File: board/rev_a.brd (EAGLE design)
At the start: 56 x 25 mm, 19 parts, among them IC3 MCP2551, Q1 35A/25V/8.5mΩ

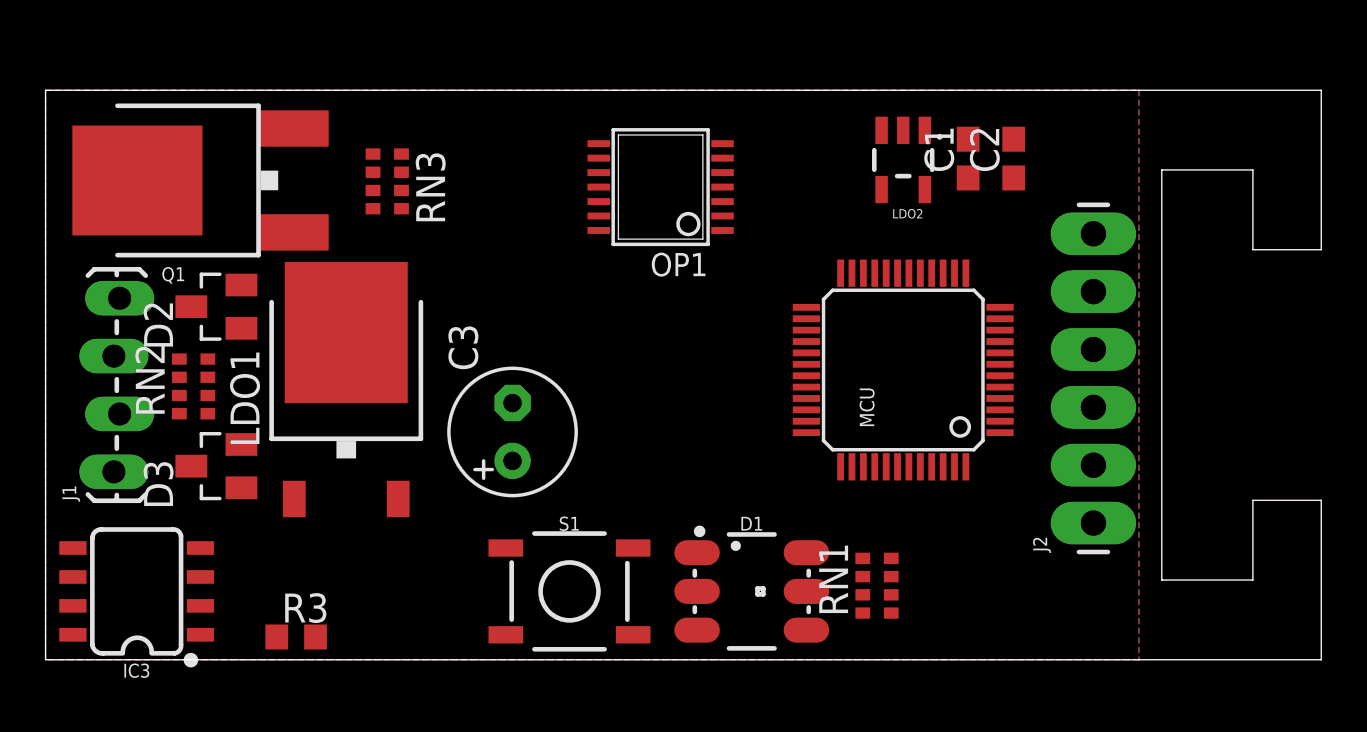
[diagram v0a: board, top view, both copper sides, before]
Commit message: [board] Testing a few configurations
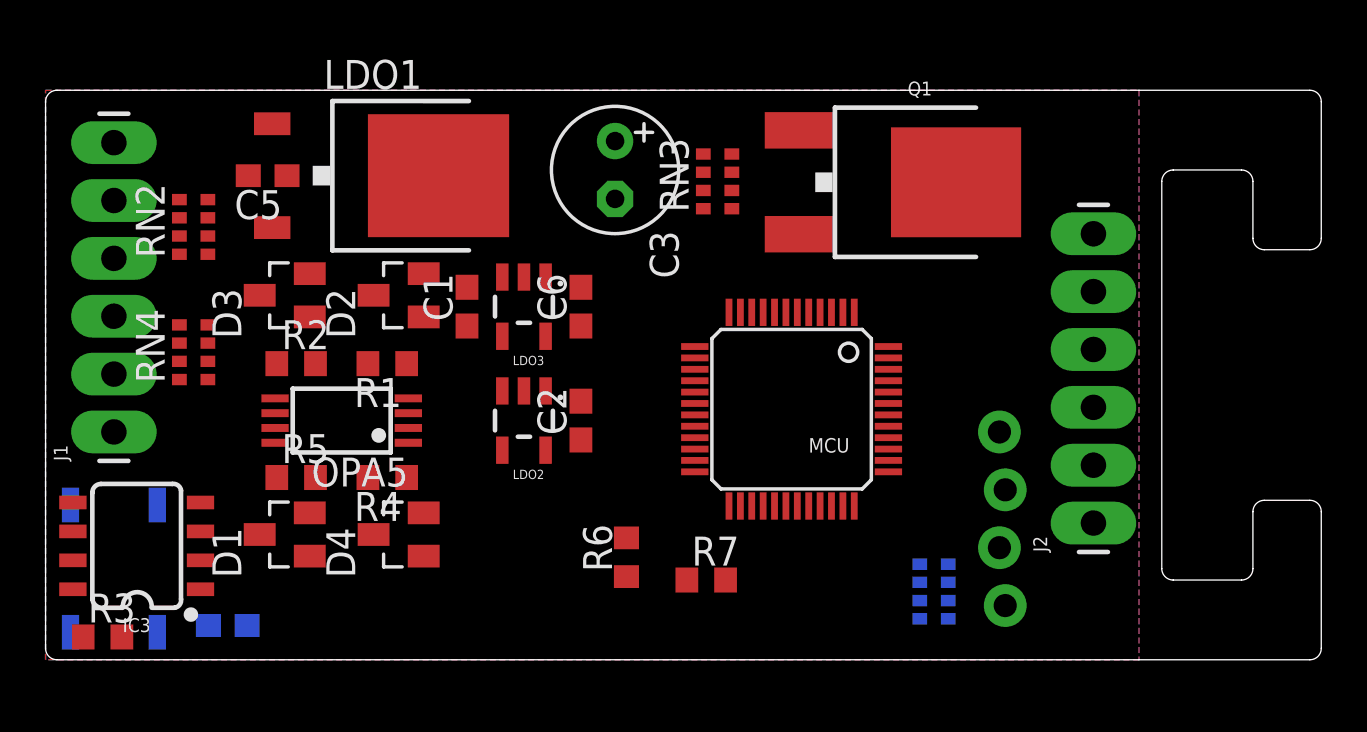
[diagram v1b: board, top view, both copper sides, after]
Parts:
- removed OP1: MCP6004, linear:TSSOP14
- added C4, C5, C6: 100nF, resistor:C0603
- added D4: BAT54S, diode:SOT23
- added J3: (no value), SparkFun-Connectors:1X04_LOCK
- added LDO3: 3.3V/150mA, SparkFun-IC-Power:SOT23-5
- added OPA5: MCP602ST, linear:TSSOP8
- added R1, R4: 20K, resistor:R0603
- added R2, R5: 10K, resistor:R0603
- added R6: 330K, resistor:R0603
- added R7: 22K, resistor:R0603
- added RN4: 1K, resistor-dil:0603-ARC
- D1: value (none) -> BAT54S; device SparkFun-LED:LED-TRICOLOR-5050 -> diode:SOT23
- J1: device SparkFun-Connectors:1X04_LOCK_LONGPADS -> SparkFun-Connectors:1X06_LONGPADS
- LDO1: value LM2936DT-5.0 -> LM2931DT-5.0
- MCU: value STM32-M-48 -> STM32F303CB
- moved Q1 32.8 mm to (38.4, 21.0), turned to 270 degrees
- moved C1 22.9 mm to (18.5, 15.5)
- moved C2 22.2 mm to (23.5, 10.5)
- moved D1 20.7 mm to (10.5, 5.50), turned to 90 degrees
- moved LDO2 20.2 mm to (21.0, 10.5)
- moved S1 20.0 mm to (3.00, 4.00), flipped to the bottom, turned to 90 degrees
- moved RN3 14.5 mm to (29.5, 21.0), turned to 270 degrees
- moved C3 12.3 mm to (25.0, 21.5), turned to 270 degrees
- moved LDO1 9.52 mm to (14.8, 21.2), turned to 270 degrees
- moved R3 8.50 mm to (2.50, 1.00)
- moved D3 8.08 mm to (10.5, 16.0)
- moved D2 8.02 mm to (15.5, 16.0)
- moved RN2 7.00 mm to (6.50, 19.0)
- moved MCU 5.19 mm to (32.8, 11.0), turned to 180 degrees
- moved RN1 2.51 mm to (39.0, 3.00), flipped to the bottom
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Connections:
- removed net N$4: C1.1, LDO2.4
- removed net TIM4_CH1: MCU.42, RN1.5
- removed net TIM4_CH2: MCU.43, RN1.7
- new net N$9: RN1.4, RN1.6
- new net OUT3: IC3.7, J1.3, RN4.1, RN4.2
- new net OUT3_PROT: D1.3, MCU.30, RN4.7, RN4.8
- new net OUT4: IC3.6, J1.2, RN4.3, RN4.4
- new net OUT4_PROT: D4.3, MCU.31, RN4.5, RN4.6
- new net SCL: J3.3, MCU.42, RN1.3
- new net SDA: J3.4, MCU.43, RN1.1
- new net VDDA: C6.1, LDO3.5, MCU.9
- net 12V: now also J1.6; no longer J1.4
- net 5V: now also C5.1, D4.2, J3.2, LDO3.1, LDO3.3, OPA5.8, RN1.5, RN1.7; no longer D1.1, D1.3, OP1.4
- net BUTTON1: now also C4.1
- net DAC1: now also OPA5.3
- net DAC2: now also OPA5.5
- net GND: now also C4.2, C5.2, C6.2, D1.1, D4.1, J3.1, LDO3.2, MCU.44, OPA5.4, R1.1, R4.1; no longer OP1.11
- net IP: now also R7.1
- net N$10: now also R6.1, R7.2; no longer OP1.7
- net N$11: now also C1.1, LDO3.4; no longer OP1.1
- net N$3: now also RN1.2, RN1.8; no longer D1.4, RN1.4
- net N$5: now also OPA5.2, R1.2, R2.2; no longer D1.6, RN1.2
- net N$6: now also R4.2, R5.2; no longer D1.5, RN1.3
- net OPA3_OUT: now also R6.2
- net OUT1: now also J1.5; no longer IC3.7, J1.3
- net OUT1_PROT: now also OPA5.1, R2.1; no longer MCU.30, OP1.8
- net OUT2: now also J1.4; no longer IC3.6, J1.2
- net OUT2_PROT: now also OPA5.7, R5.1; no longer MCU.31, OP1.14
- net TIM4_CH3: no longer RN1.6
- net VCC: no longer MCU.44, MCU.9
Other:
- outline, holes or cut-outs redrawn
